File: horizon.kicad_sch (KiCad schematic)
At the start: 25 parts, among them J2 Conn_02x03_Counter_Clockwise, J7 Conn_02x03_Counter_Clockwise, J8 Conn_02x03_Counter_Clockwise, U1 MMCU, U3 NMCU, U4 TMCU

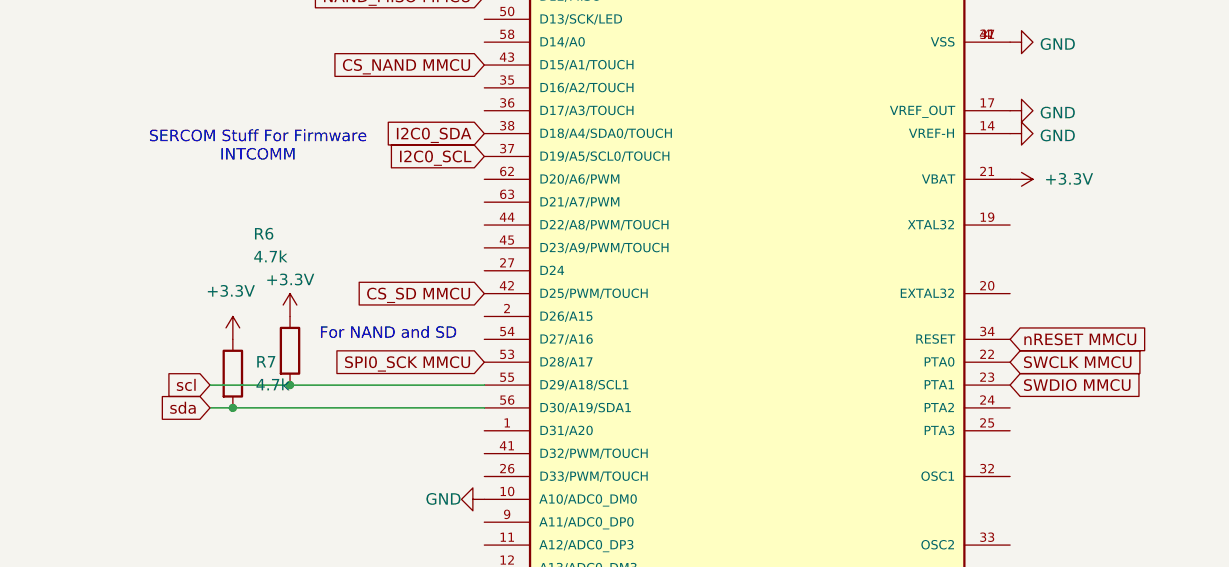
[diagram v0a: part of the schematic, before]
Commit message: misc fixes
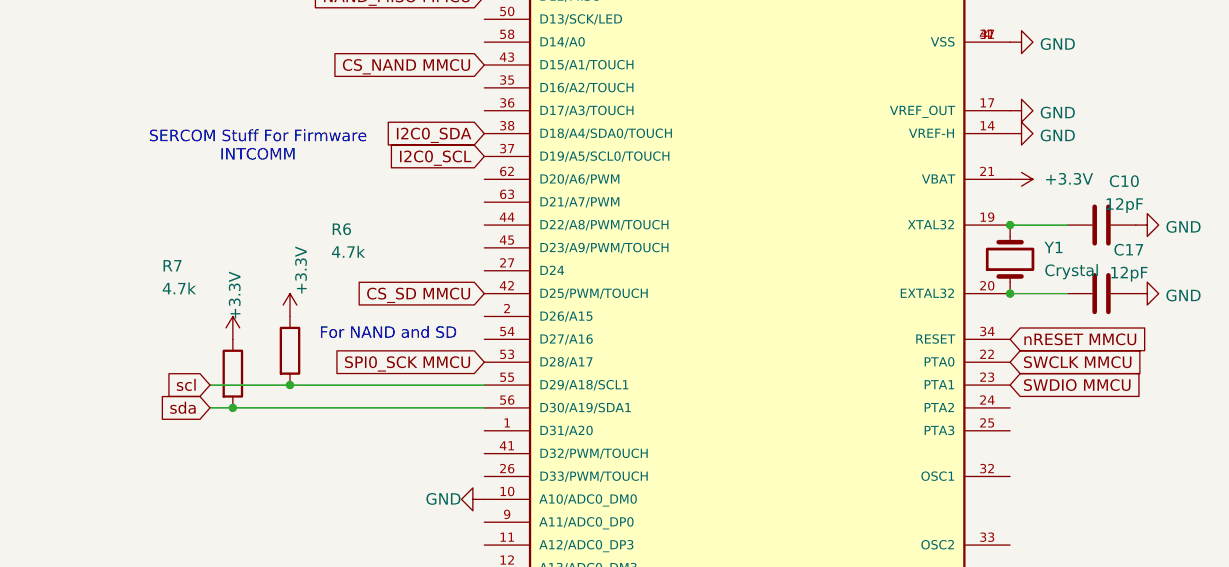
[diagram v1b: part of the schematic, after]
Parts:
- added C10, C17: 12pF, symbol Device:C
- added Y1: Crystal, symbol Device:Crystal
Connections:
- net GND: now also C10.2, C17.2
- net at U1.19 (XTAL32): now also C10.1, Y1.2
- net at U1.20 (EXTAL32): now also C17.1, Y1.1
